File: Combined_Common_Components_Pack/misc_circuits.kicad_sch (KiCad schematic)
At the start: 26 parts, among them Q10 2N7002K, Q11 2N7002K, Q9 PMOS, U8 FM8002

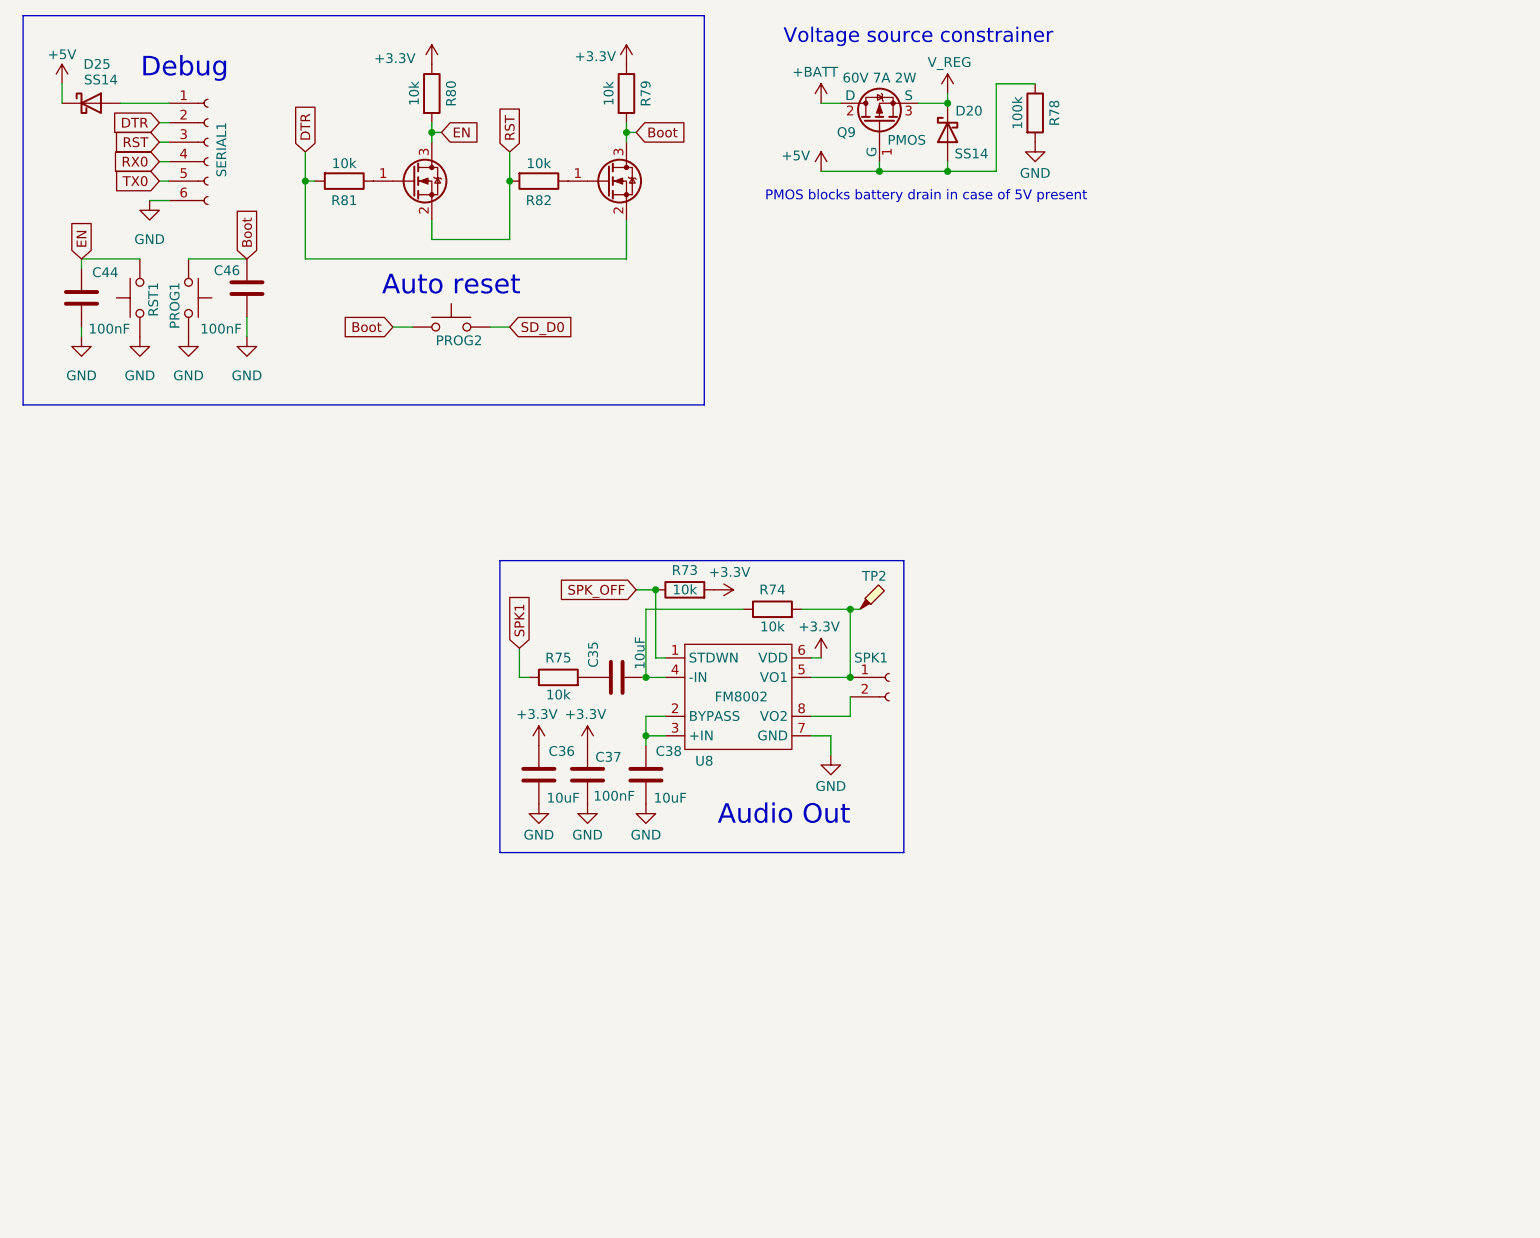
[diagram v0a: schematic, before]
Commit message: More circuits
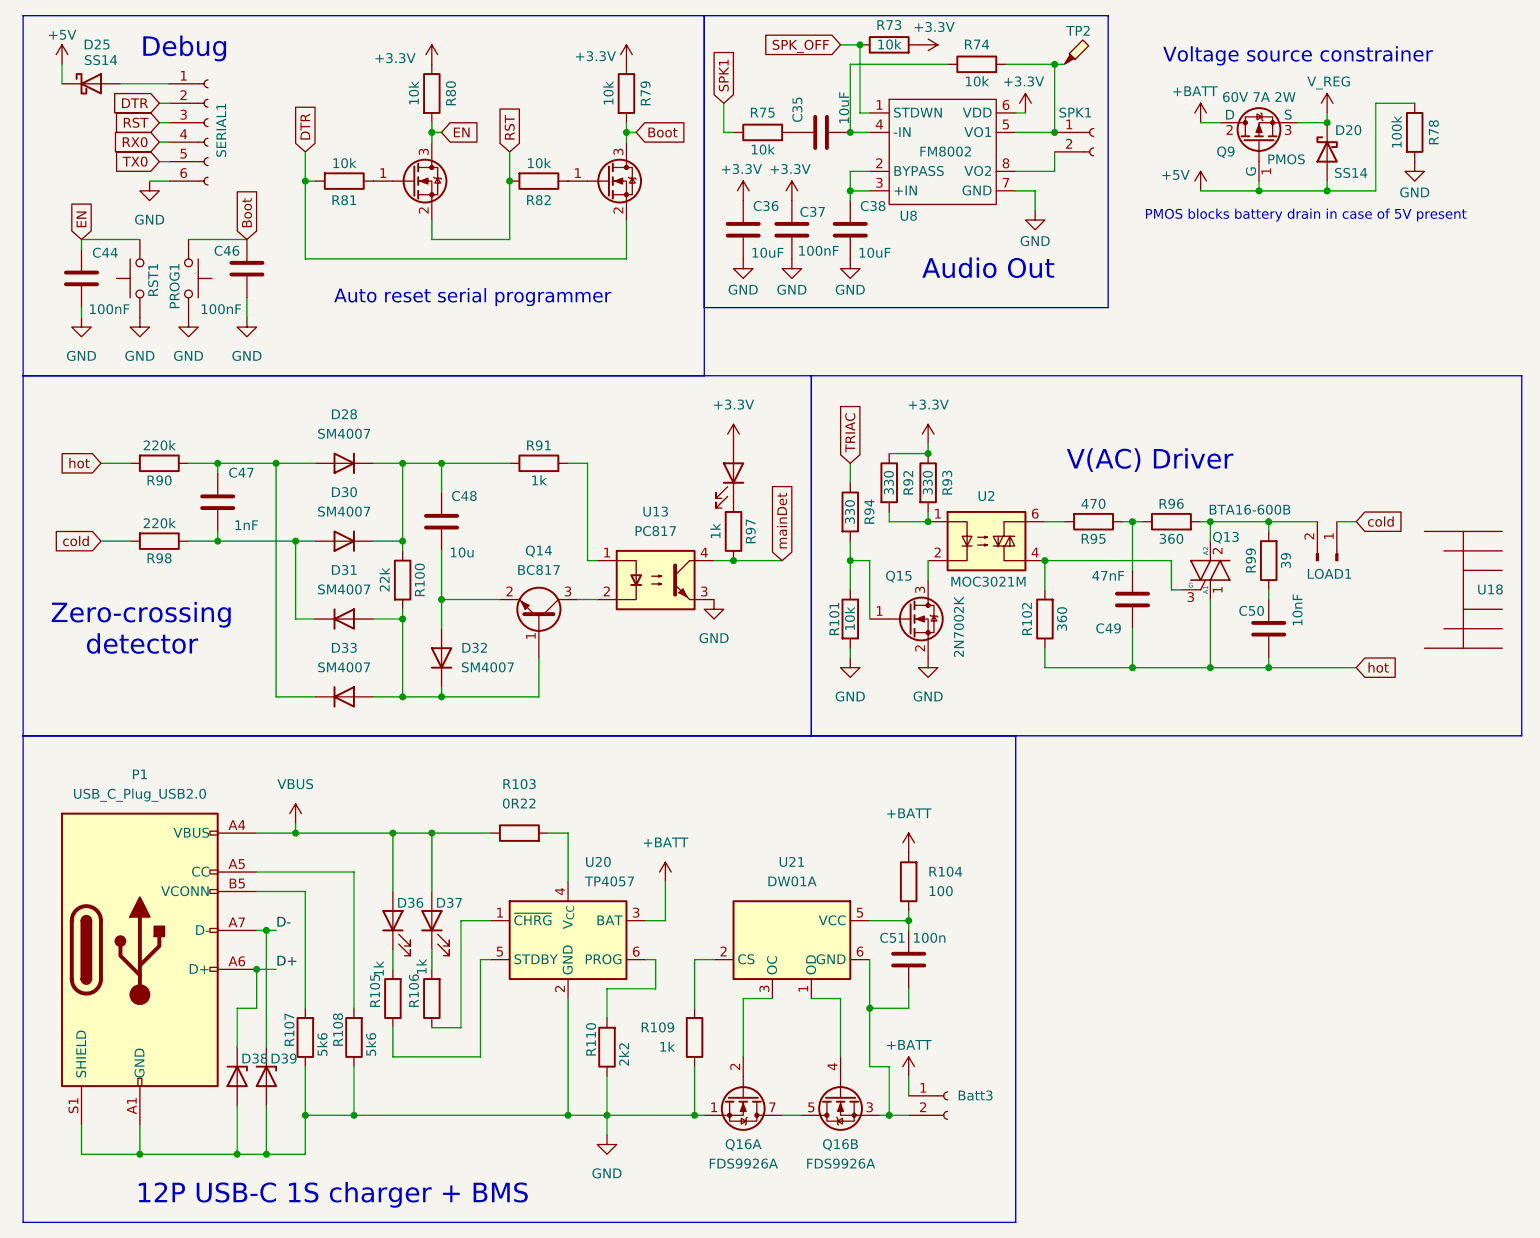
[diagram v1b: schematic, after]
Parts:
- removed PROG2: SW_Push, Button_Switch_SMD:SW_SPST_PTS647_Sx38, symbol Switch:SW_Push
- added Batt3: Conn_01x02_Socket, Connector_Molex:Molex_KK-254_AE-6410-02A_1x02_P2.54mm_Vertical, symbol Connector:Conn_01x02_Socket
- added C47: 1nF, Capacitor_SMD:C_0805_2012Metric, symbol 1_Library_GF:C_THT_RECT
- added C48: 10u, Capacitor_SMD:C_0805_2012Metric, symbol Device:C
- added C49: 47nF, Capacitor_THT:C_Rect_L11.0mm_W4.3mm_P10.00mm_MKT, symbol 1_Library_GF:C_THT_RECT
- added C50: 10nF, Capacitor_THT:C_Rect_L7.0mm_W3.5mm_P5.00mm, symbol 1_Library_GF:C_THT_RECT
- added C51: 100n, Capacitor_SMD:C_0603_1608Metric, symbol Device:C
- added D28, D30, D31, D32, D33: SM4007, Diode_SMD:D_MELF, symbol Diode:SM4007
- added D29: LED, LED_SMD:LED_0805_2012Metric_Pad1.15x1.40mm_HandSolder, symbol Device:LED
- added D36, D37: LED, LED_SMD:LED_0805_2012Metric, symbol Device:LED
- added D38, D39: PTVS5V0Z1USK, Diode_SMD:Nexperia_DSN1608-2_1.6x0.8mm, symbol Diode:PTVS5V0Z1USK
- added LOAD1: Conn_01x02_Pin, Connector_Phoenix_GMSTB:PhoenixContact_GMSTBA_2,5_2-G-7,62_1x02_P7.62mm_Horizontal, symbol Connector:Conn_01x02_Pin
- added P1: USB_C_Plug_USB2.0, Connector_USB:USB_C_Receptacle_HRO_TYPE-C-31-M-12, symbol Connector:USB_C_Plug_USB2.0
- added Q13: BTA16-600B, Package_TO_SOT_THT:TO-220-3_Vertical, symbol Triac_Thyristor:BTA16-600B
- added Q14: BC817, Package_TO_SOT_SMD:SOT-23, symbol Transistor_BJT:BC817
- added Q15: 2N7002K, Package_TO_SOT_SMD:SOT-23, symbol Transistor_FET:2N7002K
- added Q16: FDS9926A, Package_SO:SOIC-8_3.9x4.9mm_P1.27mm, symbol Transistor_FET:FDS9926A
- added R100: 22k, Resistor_SMD:R_0805_2012Metric, symbol Device:R
- added R101: 10k, Resistor_SMD:R_0805_2012Metric, symbol Device:R
- added R102, R96: 360, Resistor_THT:R_Axial_DIN0411_L9.9mm_D3.6mm_P15.24mm_Horizontal, symbol Device:R
- added R103: 0R22, Resistor_SMD:R_2010_5025Metric, symbol Device:R
- added R104: 100, Resistor_SMD:R_0603_1608Metric, symbol Device:R
- added R105, R106, R109: 1k, Resistor_SMD:R_0603_1608Metric, symbol Device:R
- added R107, R108: 5k6, Resistor_SMD:R_0603_1608Metric, symbol Device:R
- added R110: 2k2, Resistor_SMD:R_0603_1608Metric, symbol Device:R
- added R90, R98: 220k, Resistor_SMD:R_0805_2012Metric, symbol Device:R
- added R91, R97: 1k, Resistor_SMD:R_0805_2012Metric, symbol Device:R
- added R92, R93, R94: 330, Resistor_SMD:R_0805_2012Metric, symbol Device:R
- added R95: 470, Resistor_THT:R_Axial_DIN0411_L9.9mm_D3.6mm_P15.24mm_Horizontal, symbol Device:R
- added R99: 39, Resistor_THT:R_Axial_DIN0411_L9.9mm_D3.6mm_P15.24mm_Horizontal, symbol Device:R
- added U13: PC817, Package_DIP:SMDIP-4_W7.62mm, symbol Isolator:PC817
- added U18: ~, Library:HEATSINK-TH_L34.0-W12.0, symbol New_Library:Heat Sink 34X12-25
- added U2: MOC3021M, Package_DIP:SMDIP-6_W9.53mm, symbol Relay_SolidState:MOC3021M
- added U20: TP4057, Package_TO_SOT_SMD:TSOT-23-5, symbol Battery_Management:TP4057
- added U21: DW01A, Package_TO_SOT_SMD:SOT-23-6, symbol Battery_Management:DW01A
- U8: Manufacturer FM(富满) -> (none); Supplier LCSC -> (none); Supplier Part C94625 -> (none)
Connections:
- net +3.3V: now also D29.2 (A), R92.1, R93.1
- net +BATT: now also Batt3.1 (Pin_1), R104.2, U20.3 (BAT)
- net GND: now also D38.2 (A), D39.2 (A), P1.A1 (GND), P1.A12 (GND), P1.B1 (GND), P1.B12 (GND), P1.S1 (SHIELD), Q15.2 (S), Q16.1 (S1), R101.2, R107.1, R108.1, R109.1, R110.1, U13.3, U20.2 (GND)
- new net: C47.1, D30.2 (A), D31.1 (K), R98.1
- new net: D31.2 (A), D32.1 (K), D33.2 (A), Q14.1 (B), R100.2
- new net: R105.1, U20.5 (STDBY)
- new net: D36.1 (K), R105.2
- new net: LOAD1.2 (Pin_2), Q13.2 (A2), R96.2, R99.2
- new net: Q13.3 (G), R102.2, U2.4
- new net: Q15.1 (G), R101.1, R94.2
- new net: Q16.4 (G2), U21.1 (OD)
- new net: R109.2, U21.2 (CS)
- new net: Q16.2 (G1), U21.3 (OC)
- new net: C51.1, R104.1, U21.5 (VCC)
- new net: Batt3.2 (Pin_2), C51.2, Q16.3 (S2), U21.6 (GND)
- new net: C48.1, D28.1 (K), D30.1 (K), R100.1, R91.1
- new net: C47.2, D28.2 (A), D33.1 (K), R90.1
- new net: R91.2, U13.1
- new net: Q14.3 (C), U13.2
- new net: P1.B5 (VCONN), R107.2
- new net: R106.1, U20.1 (~{CHRG})
- new net: D37.1 (K), R106.2
- new net: Q16.5 (D2), Q16.6 (D2), Q16.7 (D1), Q16.8 (D1)
- new net: C50.2, R99.1
- new net: C48.2, D32.2 (A), Q14.2 (E)
- new net: R92.2, R93.2, U2.1
- new net: Q15.3 (D), U2.2
- new net: R95.2, U2.6
- new net: P1.A5 (CC), R108.2
- new net: C49.1, R95.1, R96.1
- new net: R110.2, U20.6 (PROG)
- new net: R103.2, U20.4 (V_{CC})
- new net: D29.1 (K), R97.2
- new net D+: D38.1 (K), P1.A6 (D+)
- new net D-: D39.1 (K), P1.A7 (D-)
- new net TRIAC: R94.1
- new net VBUS: D36.2 (A), D37.2 (A), P1.A4 (VBUS), P1.A9 (VBUS), P1.B4 (VBUS), P1.B9 (VBUS), R103.1
- new net cold: LOAD1.1 (Pin_1), R98.2
- new net hot: C49.2, C50.1, Q13.1 (A1), R102.1, R90.2
- new net mainDet: R97.1, U13.4
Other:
- note added: "12P USB-C 1S charger + BMS"
- note added: "Auto reset serial programmer"
- note added: "V(AC) Driver"
- note added: "Zero-crossing detector"
- note removed: "Auto reset"
- moved on the sheet: C35, C36, C37, C38, C44, C46, D20, D25, PROG1, Q9, R73, R74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
